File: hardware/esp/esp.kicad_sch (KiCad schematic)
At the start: 0 parts

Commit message: Updating PCB
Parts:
- added J1: USB_C_Receptacle_USB2.0_16P, Connector_USB:USB_C_Receptacle_HCTL_HC-TYPE-C-16P-01A, symbol Connector:USB_C_Receptacle_USB2.0_16P
- added J2: Conn_01x02, symbol Connector_Generic:Conn_01x02
- added L1: L, symbol Device:L
- added R1, R2: 22R, symbol Device:R
- added U1: BME280, Package_LGA:Bosch_LGA-8_2.5x2.5mm_P0.65mm_ClockwisePinNumbering, symbol Sensor:BME280
- added U2: VL53L0X, VL53L0X:SENSOR_VL53L0X, symbol VL53L0X:VL53L0X
- added U3: NRF24L01, Package_DFN_QFN:QFN-20-1EP_4x4mm_P0.5mm_EP2.5x2.5mm, symbol RF:NRF24L01
- added U4: ESP32-S3-WROOM-1, RF_Module:ESP32-S3-WROOM-1, symbol RF_Module:ESP32-S3-WROOM-1
- added U5: NT3H1101W0FHK, NT3H1101W0FHK:IC_NT3H1101W0FHK, symbol NT3H1101W0FHK:NT3H1101W0FHK
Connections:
- new net: U4.1 (GND), U4.40 (GND), U4.41 (GND)
- new net: L1.1, U5.8 (LB)
- new net: L1.2, U5.1 (LA)
- new net: J1.A6 (D+), J1.B6 (D+), R2.1
- new net: J1.A7 (D-), J1.B7 (D-), R1.1
- new net +5V: J1.A4 (VBUS), J1.A9 (VBUS), J1.B4 (VBUS), J1.B9 (VBUS)
- new net D+: R2.2, U4.14 (USB_D+)
- new net D-: R1.2, U4.13 (USB_D-)
- new net GND: J1.A1 (GND), J1.A12 (GND), J1.B1 (GND), J1.B12 (GND), J1.SH (SHIELD), U2.12 (GND), U2.3 (GND), U2.4 (GND), U2.6 (GND)
- new net UART_SRX: J2.2 (Pin_2)
- new net UART_STX: J2.1 (Pin_1)

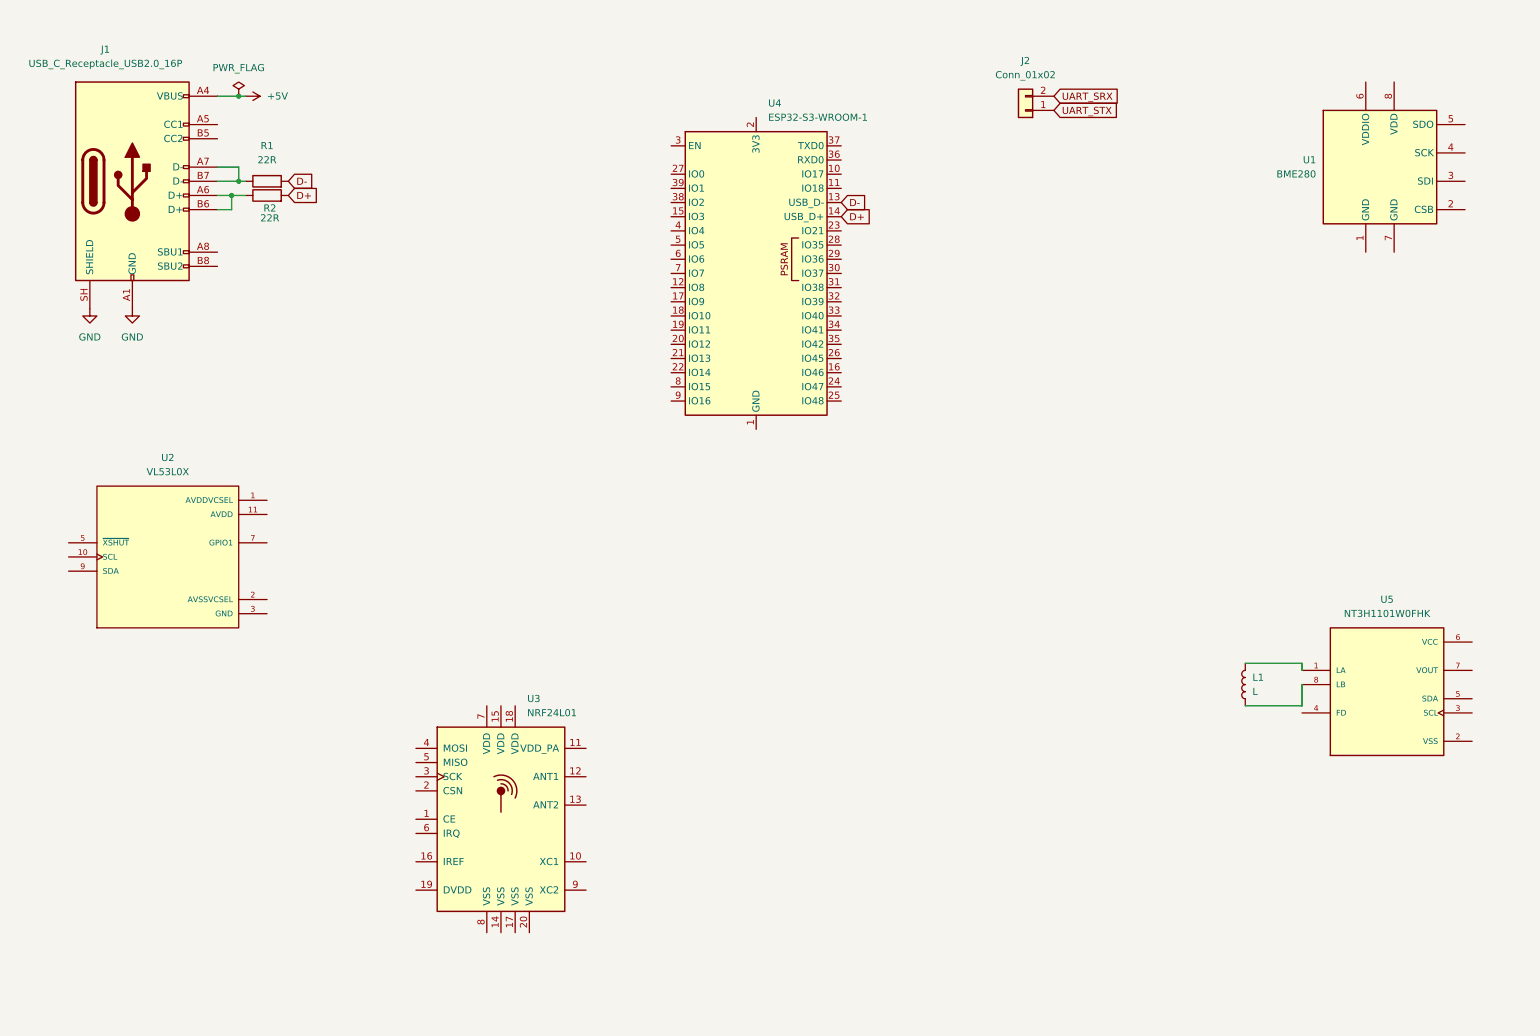
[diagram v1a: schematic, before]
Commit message: Updating schematics
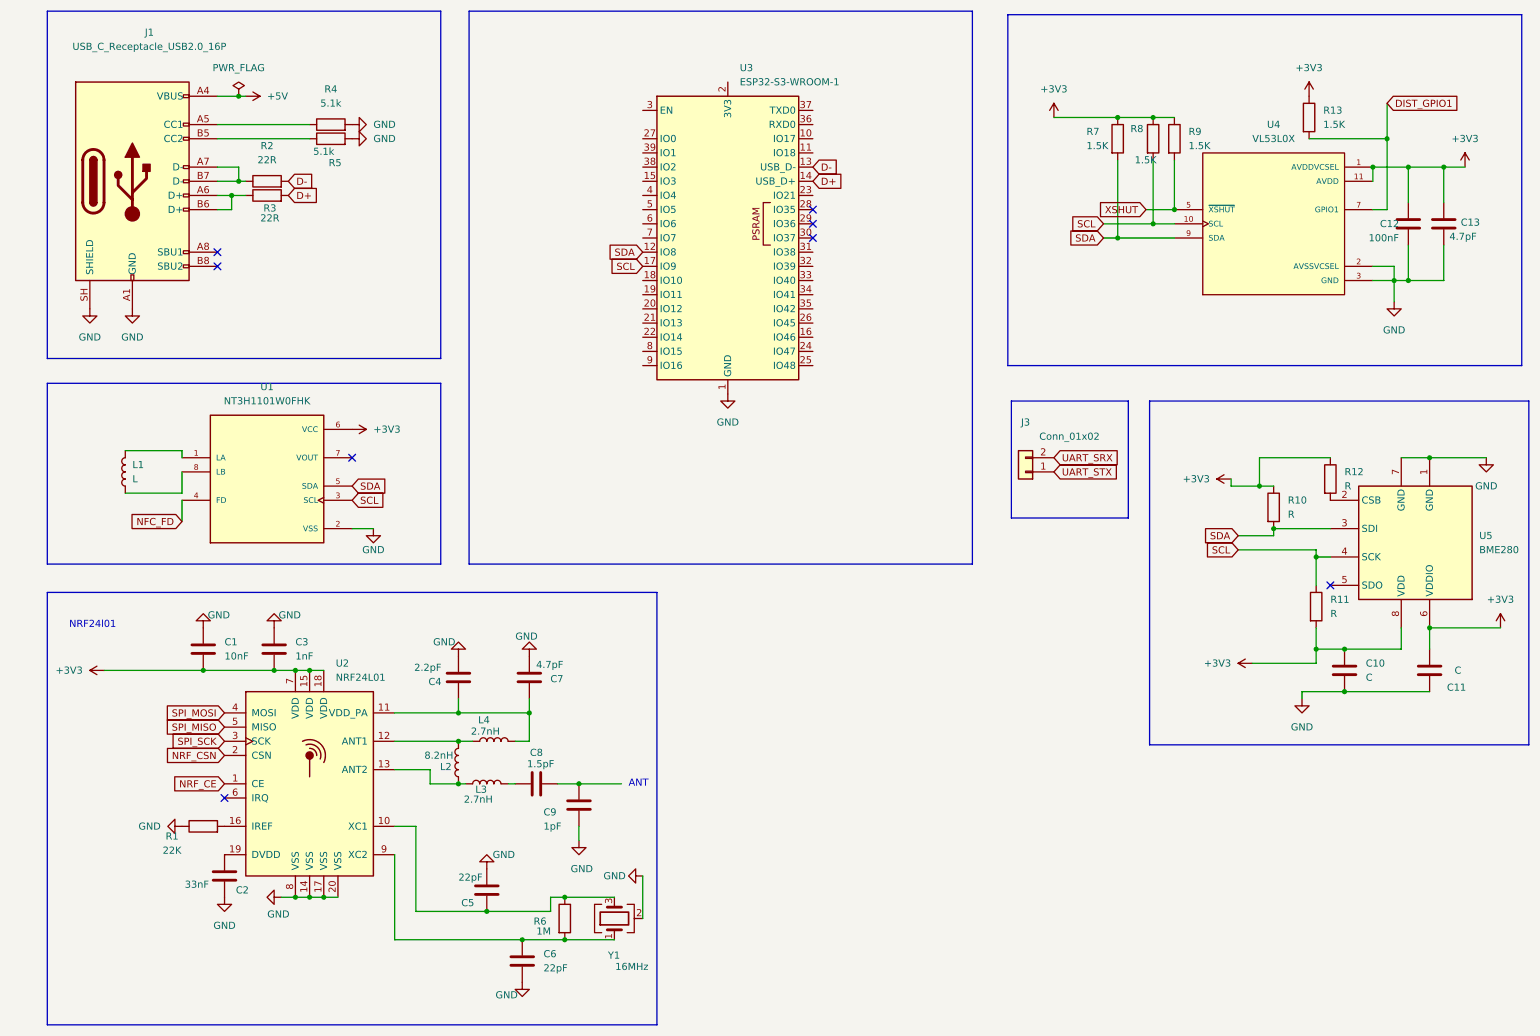
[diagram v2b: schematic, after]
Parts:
- removed U3: NRF24L01, Package_DFN_QFN:QFN-20-1EP_4x4mm_P0.5mm_EP2.5x2.5mm, symbol RF:NRF24L01
- added C1: 10nF, Capacitor_SMD:C_0603_1608Metric, symbol Device:C
- added C10, C11: C, symbol Device:C
- added C12: 100nF, symbol Device:C
- added C13: 4.7pF, symbol Device:C
- added C2: 33nF, Capacitor_SMD:C_0603_1608Metric, symbol Device:C
- added C3: 1nF, Capacitor_SMD:C_0603_1608Metric, symbol Device:C
- added C4: 2.2pF, Capacitor_SMD:C_0603_1608Metric, symbol Device:C
- added C5, C6: 22pF, Capacitor_SMD:C_0603_1608Metric, symbol Device:C
- added C7: 4.7pF, Capacitor_SMD:C_0603_1608Metric, symbol Device:C
- added C8: 1.5pF, Capacitor_SMD:C_0603_1608Metric, symbol Device:C
- added C9: 1pF, Capacitor_SMD:C_0603_1608Metric, symbol Device:C
- added L2: 8.2nH, Inductor_SMD:L_0603_1608Metric, symbol Device:L
- added L3, L4: 2.7nH, Inductor_SMD:L_0603_1608Metric, symbol Device:L
- added R1: 22K, Resistor_SMD:R_0603_1608Metric, symbol Device:R
- added R10, R11, R12: R, symbol Device:R
- added R13, R7, R8, R9: 1.5K, symbol Device:R
- added R4, R5: 5.1k, symbol Device:R
- added R6: 1M, Resistor_SMD:R_0603_1608Metric, symbol Device:R
- added U2: NRF24L01, Package_DFN_QFN:QFN-20-1EP_4x4mm_P0.5mm_EP2.5x2.5mm, symbol RF:NRF24L01
- added Y1: 16MHz, Crystal:Crystal_SMD_3225-4Pin_3.2x2.5mm, symbol Device:Crystal_GND24
- renumbered J2 to J3, R1 to R2, R2 to R3, U5 to U1, U4 to U3, U2 to U4, U1 to U5
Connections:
- net GND: now also U1.2 (VSS), U3.1 (GND), U3.40 (GND), U3.41 (GND), U4.2 (AVSSVCSEL), U5.1 (GND), U5.7 (GND), C1.1, C10.1, C11.2, C12.2, C13.2, C2.2, C3.1, C4.2, C5.1, C6.2, C7.2, C9.1, R1.1, R4.2, R5.2, U2.14 (VSS), U2.17 (VSS), U2.20 (VSS), U2.8 (VSS), Y1.2 (G), Y1.4 (G)
- net SDA: now reaches U3.12 (IO8)
- net SDA: now also U1.5 (SDA), U4.9 (SDA), U5.3 (SDI), R10.2, R7.2
- net SCL: now reaches U3.17 (IO9)
- net SCL: now also U1.3 (SCL), U4.10 (SCL), U5.4 (SCK), R11.1, R8.2
- net NFC_FD: now reaches U1.4 (FD)
- net +3V3: now reaches U1.6 (VCC)
- net +3V3: now also U4.1 (AVDDVCSEL), U4.11 (AVDD), U5.6 (VDDIO), U5.8 (VDD), C1.2, C10.2, C11.1, C12.1, C13.1, C3.2, R10.1, R11.2, R12.1, R13.1, R7.1, R8.1, R9.1, U2.15 (VDD), U2.18 (VDD), U2.7 (VDD)
- net XSHUT: now reaches U4.5 (~{XSHUT})
- net XSHUT: now also R9.2
- net DIST_GPIO1: now reaches U4.7 (GPIO1)
- net DIST_GPIO1: now also R13.2
- net at U5.2 (CSB): now also R12.2
- net at J1.A5 (CC1): now also R4.1
- net at J1.B5 (CC2): now also R5.1
- new net: C8.1, L3.2
- new net: C8.2, C9.2
- new net: L2.1, L3.1, U2.13 (ANT2)
- new net: C4.1, C7.1, L4.2, U2.11 (VDD_PA)
- new net: C5.2, R6.1, U2.10 (XC1), Y1.3
- new net: C6.1, R6.2, U2.9 (XC2), Y1.1
- new net: L2.2, L4.1, U2.12 (ANT1)
- new net: R1.2, U2.16 (IREF)
- new net: C2.1, U2.19 (DVDD)
- new net NRF_CE: U2.1 (CE)
- new net NRF_CSN: U2.2 (CSN)
- new net SPI_MISO: U2.5 (MISO)
- new net SPI_MOSI: U2.4 (MOSI)
- new net SPI_SCK: U2.3 (SCK)
- no-connect marks 0 -> 8
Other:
- note added: "ANT"
- note added: "NRF24l01"
- moved on the sheet: J3, L1, U1, U3, U4, U5

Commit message: Updating PCb and esp board schematics
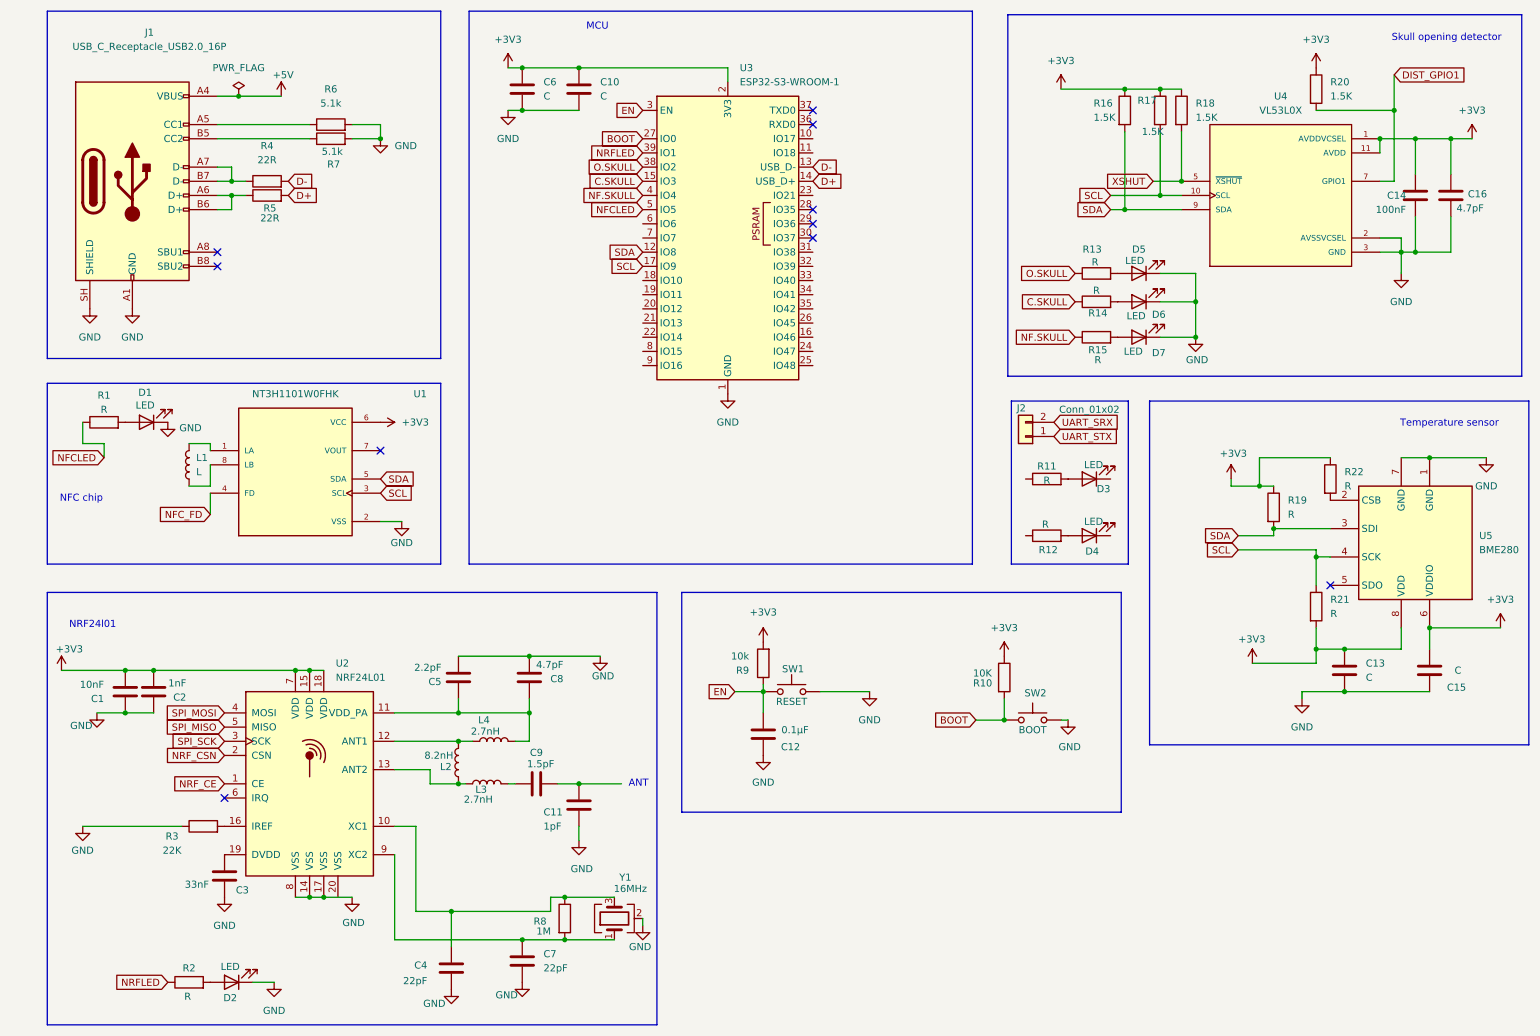
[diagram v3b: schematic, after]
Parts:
- added C10, C6: C, symbol Device:C
- added C12: 0.1µF, Capacitor_SMD:C_0805_2012Metric, symbol Device:C
- added D1, D2, D3, D4, D5, D6, D7: LED, symbol Device:LED
- added R1, R11, R12, R13, R14, R15, R2: R, symbol Device:R
- added R10: 10K, Resistor_SMD:R_0805_2012Metric, symbol Device:R
- added R9: 10k, Resistor_SMD:R_0805_2012Metric, symbol Device:R
- added SW1: RESET, Button_Switch_SMD:SW_SPST_SKQG_WithStem, symbol Switch:SW_Push
- added SW2: BOOT, Button_Switch_SMD:SW_SPST_SKQG_WithStem, symbol Switch:SW_Push
- C13: renamed from C10; footprint (none) -> Capacitor_SMD:C_0603_1608Metric
- C14: renamed from C12; footprint (none) -> Capacitor_SMD:C_0603_1608Metric
- C15: renamed from C11; footprint (none) -> Capacitor_SMD:C_0603_1608Metric
- C16: renamed from C13; footprint (none) -> Capacitor_SMD:C_0603_1608Metric
- R16: renamed from R7; footprint (none) -> Resistor_SMD:R_0805_2012Metric
- R17: renamed from R8; footprint (none) -> Resistor_SMD:R_0805_2012Metric
- R18: renamed from R9; footprint (none) -> Resistor_SMD:R_0805_2012Metric
- R19: renamed from R10; footprint (none) -> Resistor_SMD:R_0805_2012Metric
- R20: renamed from R13; footprint (none) -> Resistor_SMD:R_0805_2012Metric
- R21: renamed from R11; footprint (none) -> Resistor_SMD:R_0805_2012Metric
- R22: renamed from R12; footprint (none) -> Resistor_SMD:R_0805_2012Metric
- R4: renamed from R2; footprint (none) -> Resistor_SMD:R_0805_2012Metric
- R5: renamed from R3; footprint (none) -> Resistor_SMD:R_0805_2012Metric
- R6: renamed from R4; footprint (none) -> Resistor_SMD:R_0805_2012Metric
- R7: renamed from R5; footprint (none) -> Resistor_SMD:R_0805_2012Metric
- R8: renamed from R6; footprint Resistor_SMD:R_0603_1608Metric -> Resistor_SMD:R_0805_2012Metric
- renumbered C9 to C11, C3 to C2, C2 to C3, C5 to C4, C4 to C5, C6 to C7, C7 to C8, C8 to C9, J3 to J2, R1 to R3
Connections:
- net +3V3: now also U3.2 (3V3), C10.2, C6.2, R10.1, R9.2
- net GND: now also C10.1, C12.1, C6.1, D1.1 (K), D2.1 (K), D5.1 (K), D6.1 (K), D7.1 (K), SW1.2, SW2.2; no longer U2.20 (VSS)
- net C.SKULL: now reaches U3.15 (IO3)
- net C.SKULL: now also R14.1
- net BOOT: now reaches U3.27 (IO0)
- net BOOT: now also R10.2, SW2.1
- net EN: now reaches U3.3 (EN)
- net EN: now also C12.2, R9.1, SW1.1
- net O.SKULL: now reaches U3.38 (IO2)
- net O.SKULL: now also R13.1
- net NRFLED: now reaches U3.39 (IO1)
- net NRFLED: now also R2.1
- net NF.SKULL: now reaches U3.4 (IO4)
- net NF.SKULL: now also R15.1
- net NFCLED: now reaches U3.5 (IO5)
- net NFCLED: now also R1.1
- new net: D7.2 (A), R15.2
- new net: D2.2 (A), R2.2
- new net: D3.2 (A), R11.2
- new net: D5.2 (A), R13.2
- new net: D1.2 (A), R1.2
- new net: D4.2 (A), R12.2
- new net: D6.2 (A), R14.2
- no-connect marks 8 -> 10
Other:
- note added: "MCU"
- note added: "NFC chip"
- note added: "Skull opening detector"
- note added: "Temperature sensor"
- moved on the sheet: C1, C14, C16, C2, C4, J2, L1, R16, R17, R18, R20, U1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
